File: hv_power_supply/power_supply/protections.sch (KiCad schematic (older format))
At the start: 15 parts, among them K2 LI12-1A85(NO), Q2 SSM3K333R

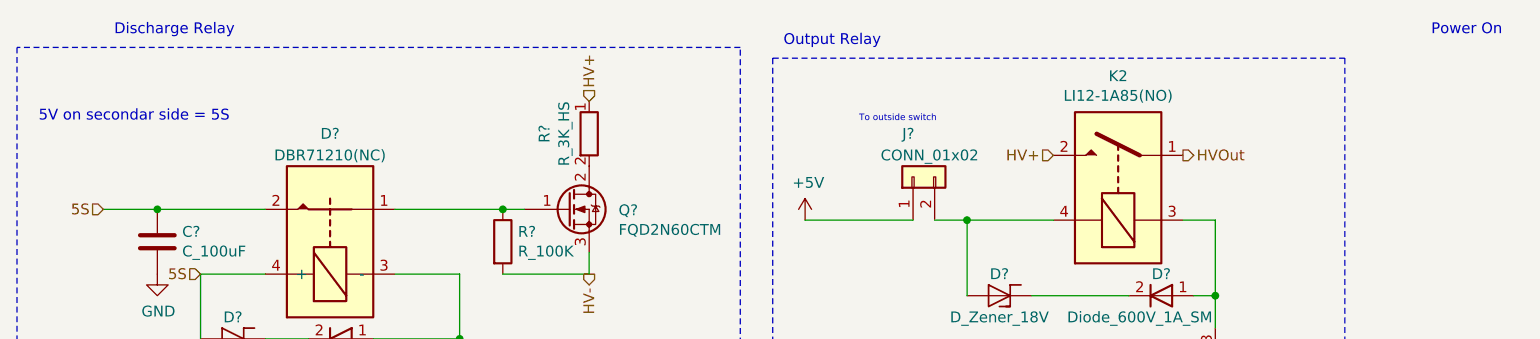
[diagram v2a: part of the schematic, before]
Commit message: minor change
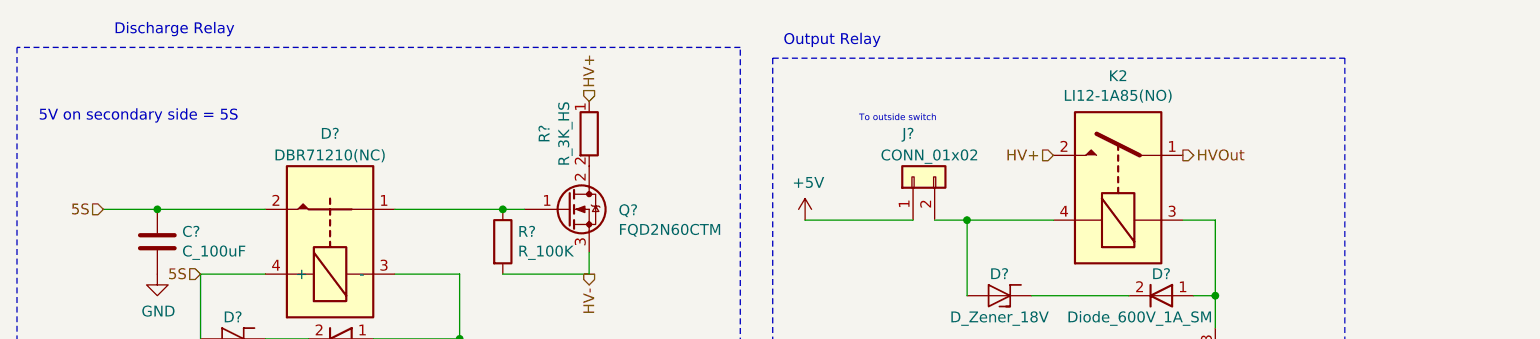
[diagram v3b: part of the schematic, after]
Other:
- note added: "5V on secondary side = 5S"
- note removed: "5V on secondar side = 5S"
- note removed: "Power On"
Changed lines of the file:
@@
 	2650 2150 2650 2400
 Text Notes 700  1150 0    50   ~ 0
-5V on secondar side = 5S
+5V on secondary side = 5S
 Wire Wire Line
 	1000 1550 1250 1550
@@
 Wire Notes Line
 	600  800  600  3150
-Text Notes 7150 750  0    50   ~ 0
-Power On
 $EndSCHEMATC
